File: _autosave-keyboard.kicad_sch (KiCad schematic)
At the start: 14 parts, among them SW1 SW_Push, U1 ATmega32U4-A, Y1 16 MHz

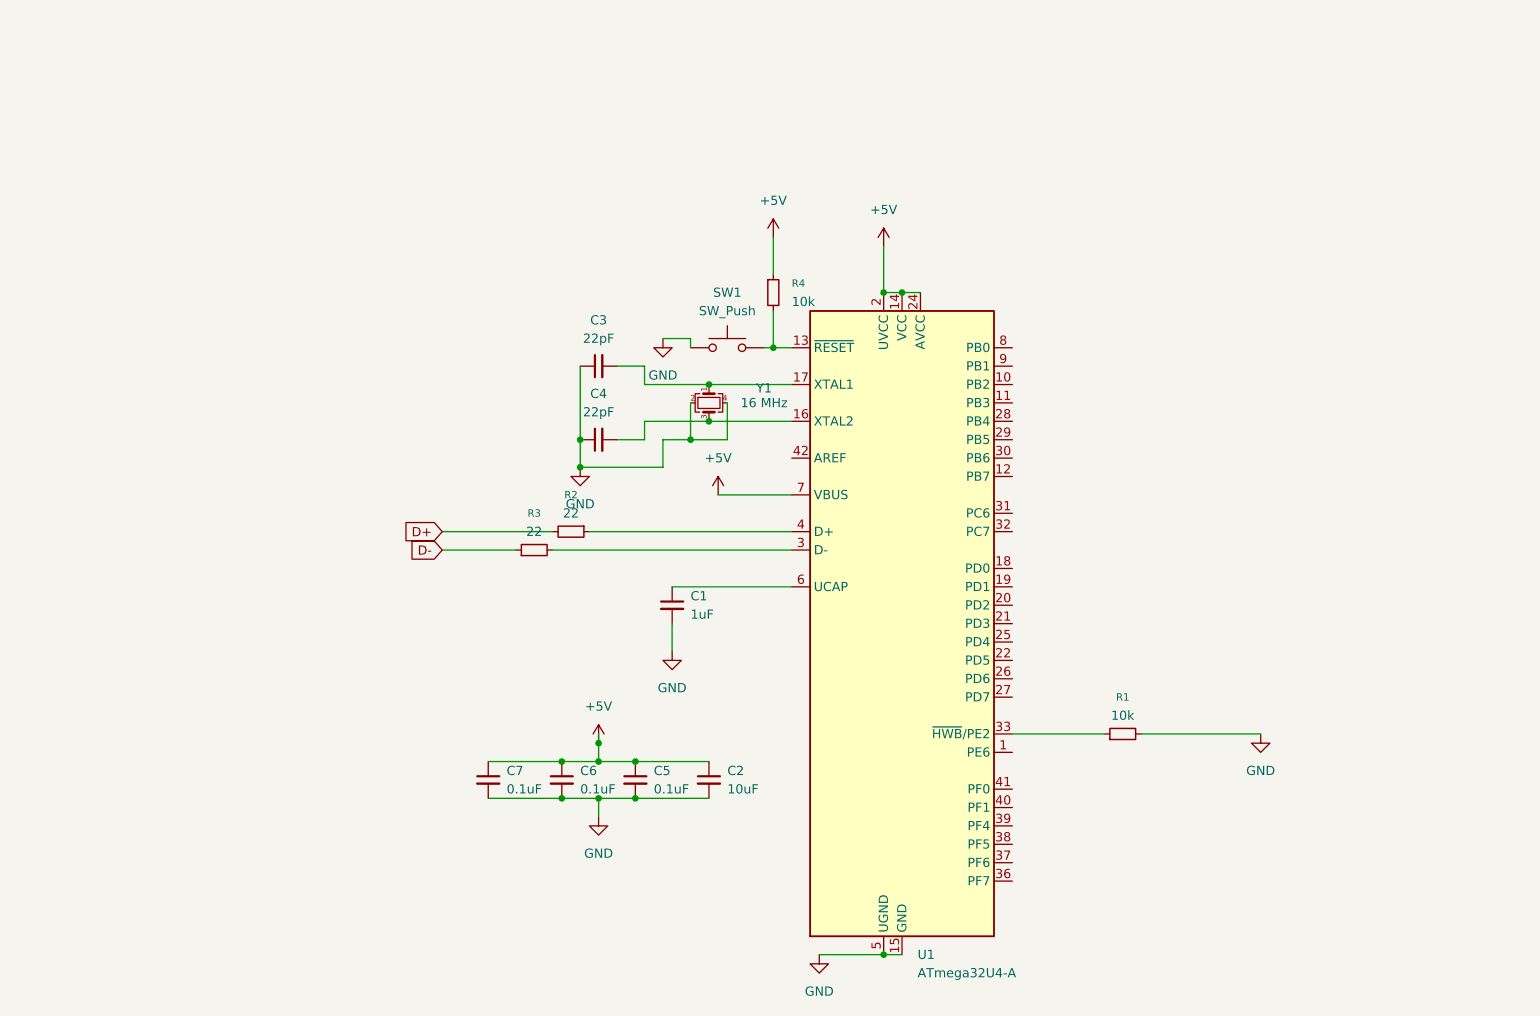
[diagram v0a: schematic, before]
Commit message: idk man, i'm just following the tutorial
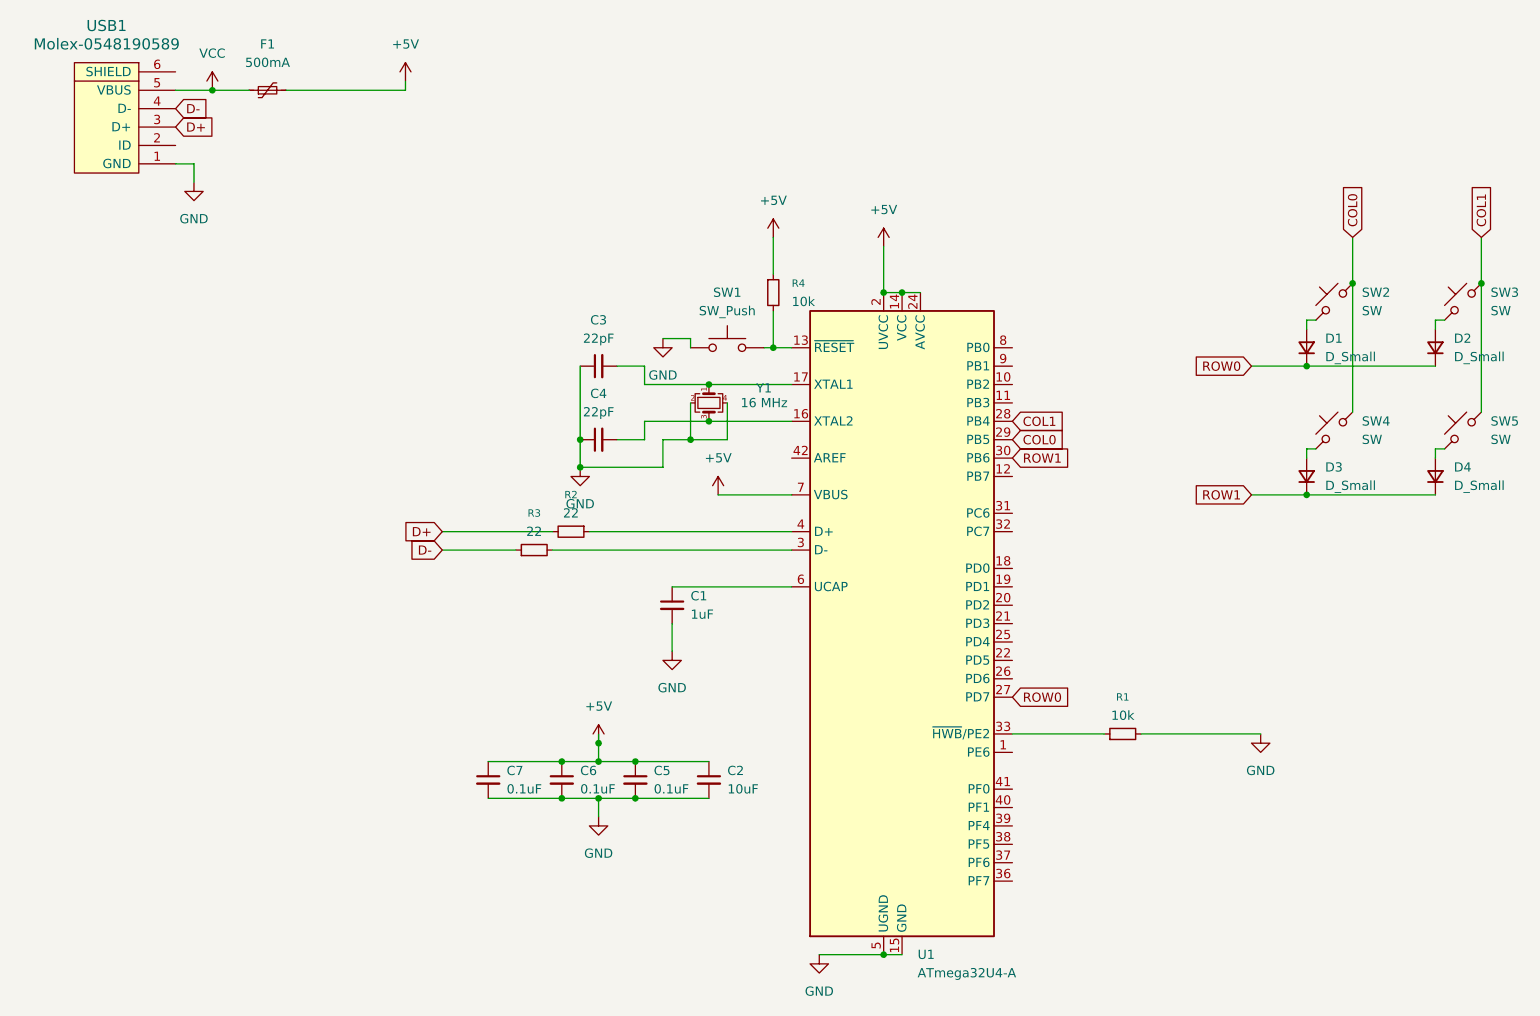
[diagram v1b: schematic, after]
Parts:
- added D1, D2, D3, D4: D_Small, symbol Device:D_Small
- added F1: 500mA, symbol Device:Polyfuse_Small
- added SW2, SW3, SW4, SW5: SW, key-switches:SW_Gateron_LowProfile_THT, symbol Switch:SW_Push_45deg
- added USB1: Molex-0548190589, symbol random-keyboard-parts:Molex-0548190589
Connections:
- net +5V: now also F1.2
- net D+: now also USB1.3 (D+)
- net D-: now also USB1.4 (D-)
- net GND: now also USB1.1 (GND)
- net ROW0: now reaches U1.27 (PD7)
- net ROW0: now also D1.1 (K), D2.1 (K)
- net COL1: now reaches U1.28 (PB4)
- net COL1: now also SW3.2, SW5.2
- net COL0: now reaches U1.29 (PB5)
- net COL0: now also SW2.2, SW4.2
- net ROW1: now reaches U1.30 (PB6)
- net ROW1: now also D3.1 (K), D4.1 (K)
- new net: D4.2 (A), SW5.1
- new net: D1.2 (A), SW2.1
- new net: D3.2 (A), SW4.1
- new net: D2.2 (A), SW3.1
- new net VCC: F1.1, USB1.5 (VBUS)
